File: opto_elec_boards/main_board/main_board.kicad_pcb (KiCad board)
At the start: 2 copper layers, 216.5 x 68.6 mm, 19 parts, among them J1 IN1_BNC, J2 IN2_BNC, J3 OUT1_BNC, J4 OUT2_BNC, J5 OUT3_BNC, J6 OUT4_BNC, J7 Conn_01x02, J8 Conn_01x02, J9 Conn_01x18, U1 L7805, U2 L78L33_TO92

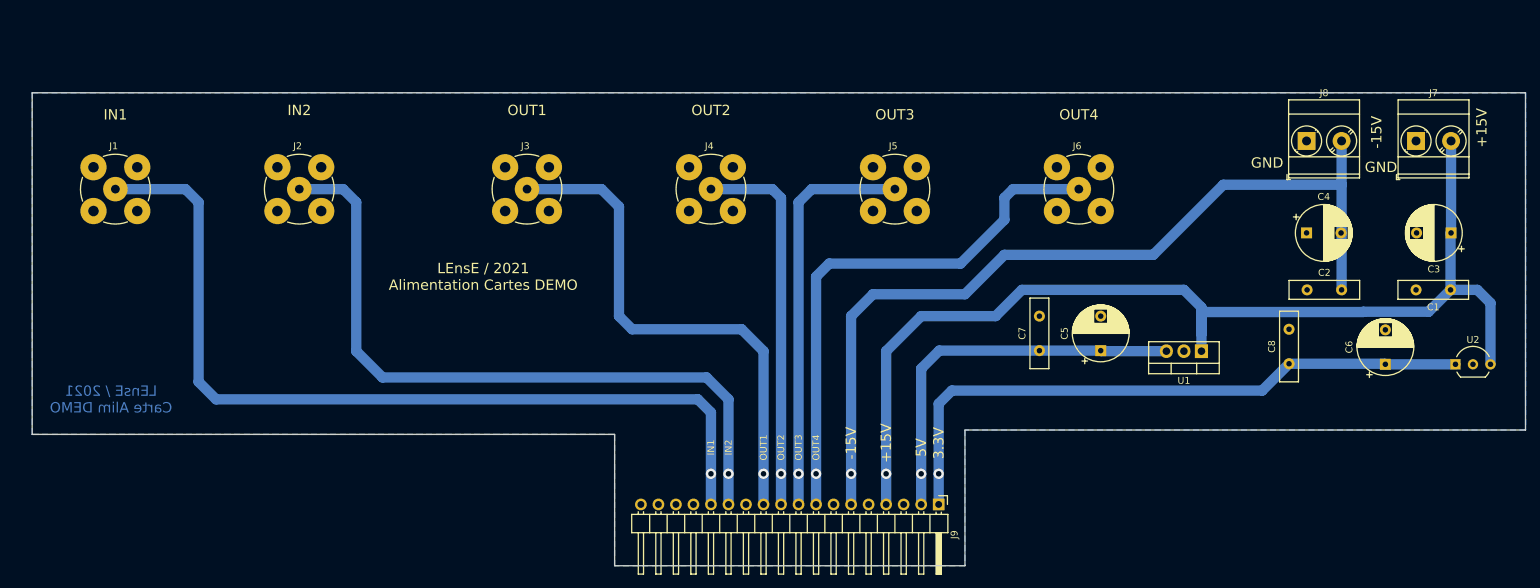
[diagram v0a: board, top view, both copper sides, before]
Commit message: Update OptoElec Board / Main board
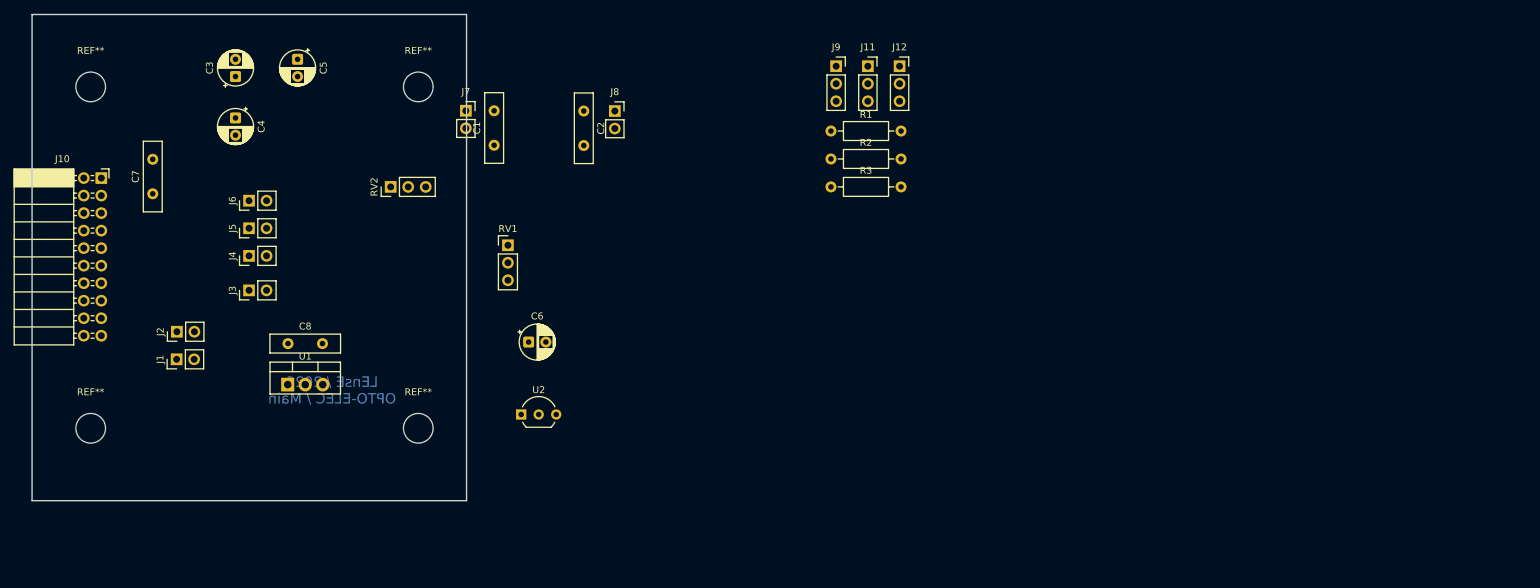
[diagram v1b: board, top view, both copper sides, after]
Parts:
- added J10: To Slave Board, Connector_PinSocket_2.54mm:PinSocket_2x10_P2.54mm_Horizontal, F.Cu at (66.5, 58.7)
- added J11: SWITCH_B, Connector_PinSocket_2.54mm:PinSocket_1x03_P2.54mm_Vertical, F.Cu at (177.7, 42.5)
- added J12: SWITCH_C, Connector_PinSocket_2.54mm:PinSocket_1x03_P2.54mm_Vertical, F.Cu at (182.3, 42.5)
- added R1: 8.2k, Resistor_THT:R_Axial_DIN0207_L6.3mm_D2.5mm_P10.16mm_Horizontal, F.Cu at (172.3, 51.9)
- added R2: 8.2k, Resistor_THT:R_Axial_DIN0207_L6.3mm_D2.5mm_P10.16mm_Horizontal, F.Cu at (172.3, 56.0)
- added R3: 8.2k, Resistor_THT:R_Axial_DIN0207_L6.3mm_D2.5mm_P10.16mm_Horizontal, F.Cu at (172.3, 60.0)
- added REF**: MountingHole_4.3mm_M4, MountingHole:MountingHole_4.3mm_M4, F.Cu at (65.0, 45.5)
- added REF**: MountingHole_4.3mm_M4, MountingHole:MountingHole_4.3mm_M4, F.Cu at (65.0, 95.0)
- added REF**: MountingHole_4.3mm_M4, MountingHole:MountingHole_4.3mm_M4, F.Cu at (112.5, 95.0)
- added REF**: MountingHole_4.3mm_M4, MountingHole:MountingHole_4.3mm_M4, F.Cu at (112.5, 45.5)
- added RV1: R_Potentiometer, Connector_PinHeader_2.54mm:PinHeader_1x03_P2.54mm_Vertical, F.Cu at (125.5, 68.5)
- added RV2: R_Potentiometer, Connector_PinHeader_2.54mm:PinHeader_1x03_P2.54mm_Vertical, F.Cu at (108.5, 60.0)
- C3, C4, C5, C6: value 10u -> 10uF; footprint Capacitor_THT:CP_Radial_D8.0mm_P5.00mm -> Capacitor_THT:CP_Radial_D5.0mm_P2.50mm
- J1, J2, J3, J4, J5, J6: footprint Connector_Coaxial:BNC_TEConnectivity_1478204_Vertical -> Connector_PinHeader_2.54mm:PinHeader_1x02_P2.54mm_Vertical
- J7: value Conn_01x02 -> POW_+15V; footprint TerminalBlock_Phoenix:TerminalBlock_Phoenix_MKDS-3-2-5.08_1x02_P5.08mm_Horizontal -> Connector_PinSocket_2.54mm:PinSocket_1x02_P2.54mm_Vertical
- J8: value Conn_01x02 -> POW_-15V; footprint TerminalBlock_Phoenix:TerminalBlock_Phoenix_MKDS-3-2-5.08_1x02_P5.08mm_Horizontal -> Connector_PinSocket_2.54mm:PinSocket_1x02_P2.54mm_Vertical
- J9: value Conn_01x18 -> SWITCH_A; footprint Connector_PinHeader_2.54mm:PinHeader_1x18_P2.54mm_Horizontal -> Connector_PinSocket_2.54mm:PinSocket_1x03_P2.54mm_Vertical
- moved C3 177.7 mm to (86.0, 44.0), turned to 90 degrees
- moved C4 156.2 mm to (86.0, 50.0), turned to -90 degrees
- moved C8 145.2 mm to (93.6, 82.7), turned to 0 degrees
- moved C1 140.3 mm to (123.5, 54.0), turned to 90 degrees
- moved J7 137.8 mm to (119.4, 49.0)
- moved U2 135.7 mm to (127.4, 93.0)
- moved U1 132.6 mm to (93.6, 88.7), turned to 0 degrees
- moved C7 130.6 mm to (74.0, 61.0)
- moved C6 124.3 mm to (128.5, 82.5), turned to 0 degrees
- moved C5 123.9 mm to (95.0, 41.5), turned to -90 degrees
- moved J6 120.3 mm to (88.0, 62.0), turned to 90 degrees
- moved C2 108.0 mm to (136.5, 49.0), turned to -90 degrees
- moved J8 100.4 mm to (141.0, 49.0)
- moved J5 93.8 mm to (88.0, 66.0), turned to 90 degrees
- moved J4 67.7 mm to (88.0, 70.0), turned to 90 degrees
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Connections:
- C4 pad 1: GND -> 5V
- C4 pad 2: -15V -> GND
- C5 pad 1: 5V -> GND
- C5 pad 2: GND -> -15V
- J9 pad 1: 3.3V -> GND
- J9 pad 2: 5V -> SEL1
- J9 pad 3: GND -> 3.3V
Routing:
- net +15V: track 156.8 -> 0.00 mm, vias 1 -> 0
- net IN1: track 128.4 -> 0.00 mm, vias 1 -> 0
- net -15V: track 128.0 -> 0.00 mm, vias 1 -> 0
- net IN2: track 102.7 -> 0.00 mm, vias 1 -> 0
- net 3.3V: track 92.0 -> 0.00 mm, vias 1 -> 0
- net OUT4: track 78.2 -> 0.00 mm, vias 1 -> 0
- net OUT1: track 75.5 -> 0.00 mm, vias 1 -> 0
- net OUT3: track 58.6 -> 0.00 mm, vias 1 -> 0
- net 5V: track 56.4 -> 0.00 mm, vias 1 -> 0
- net OUT2: track 55.1 -> 0.00 mm, vias 1 -> 0
- removed copper zone on B.Cu, net GND
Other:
- board size 216.5 x 68.6 mm -> 63 x 70.5 mm
- net class Default removed
- board text added: "LEnsE / 2026 OPTO-ELEC / Main"
- board text removed: "+15V"
- board text removed: "-15V"
- board text removed: "3.3V"
- board text removed: "5V"
- board text removed: "GND"
- board text removed: "IN1"
- board text removed: "IN2"
- board text removed: "LEnsE / 2021 Alimentation Cartes DEMO"
- board text removed: "LEnsE / 2021 Carte Alim DEMO"
- board text removed: "OUT1"
- board text removed: "OUT2"
- board text removed: "OUT3"
- board text removed: "OUT4"
